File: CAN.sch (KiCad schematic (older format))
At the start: 9 parts, among them U7 MCP2542FDxMF

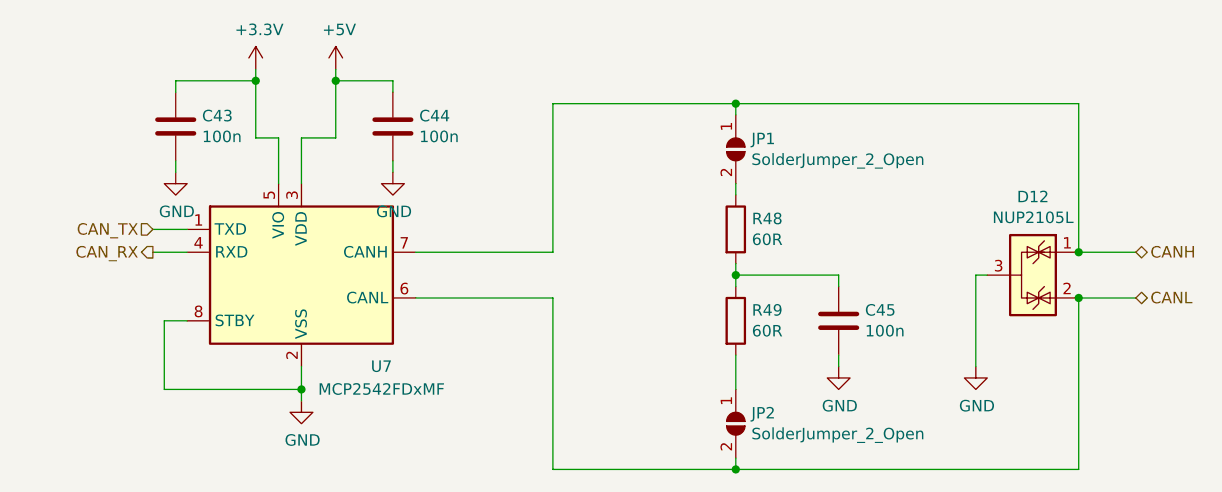
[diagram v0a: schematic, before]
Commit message: Added FET for LED
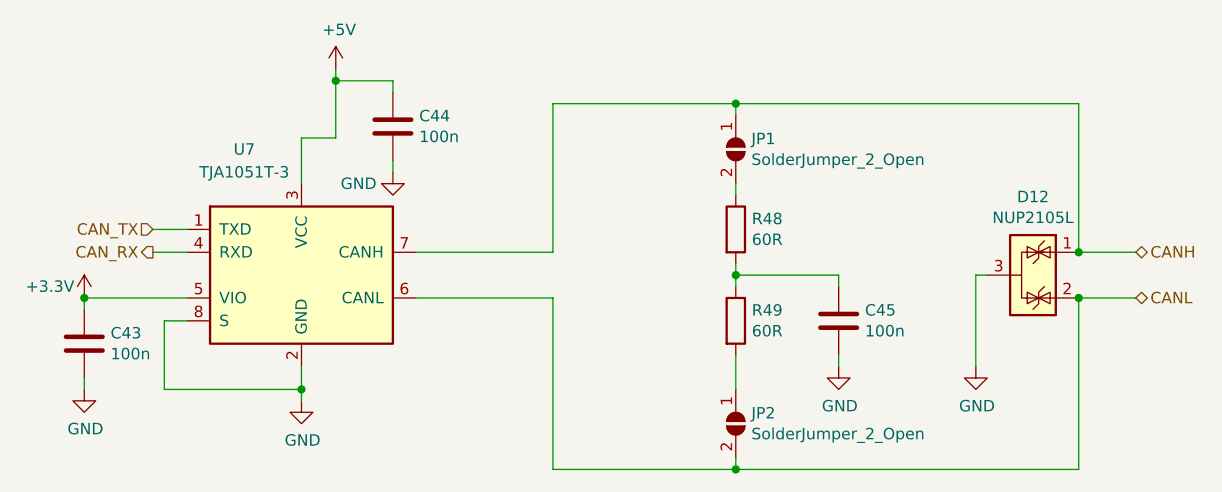
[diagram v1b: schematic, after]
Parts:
- removed U7: MCP2542FDxMF, Package_DFN_QFN:DFN-8-1EP_3x3mm_P0.65mm_EP1.55x2.4mm, symbol Interface_CAN_LIN:MCP2542FDxMF
- added U7: TJA1051T-3, Package_SO:SOIC-8_3.9x4.9mm_P1.27mm, symbol Interface_CAN_LIN:TJA1051T-3
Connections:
- net +3V3: now also U7.5 (VIO)
- net +5V: now also U7.3 (VCC)
- net CANH: now also U7.7 (CANH)
- net CANL: now also U7.6 (CANL)
- net CAN_RX: now also U7.4 (RXD)
- net CAN_TX: now also U7.1 (TXD)
- net GND: now also U7.2 (GND), U7.8 (S)
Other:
- moved on the sheet: C43
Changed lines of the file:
@@
 Comment4 ""
 $EndDescr
-$Comp
-L Interface_CAN_LIN:MCP2542FDxMF U7
-U 1 1 5F738629
-P 4750 3600
-F 0 "U7" H 5100 3200 50  0000 C CNN
-F 1 "MCP2542FDxMF" H 5100 3100 50  0000 C CNN
-F 2 "Package_DFN_QFN:DFN-8-1EP_3x3mm_P0.65mm_EP1.55x2.4mm" H 4750 3100 50  0001 C CIN
-F 3 "http://ww1.microchip.com/downloads/en/DeviceDoc/MCP2542FD-4FD-MCP2542WFD-4WFD-Data-Sheet20005514B.pdf" H 4750 3600 50  0001 C CNN
-	1    4750 3600
-	1    0    0    -1
-$EndComp
 Wire Wire Line
 	5250 3500 5850 3500
@@
 L power:+3.3V #PWR0228
 U 1 1 5F74847C
-P 4550 2700
-F 0 "#PWR0228" H 4550 2550 50  0001 C CNN
-F 1 "+3.3V" H 4565 2873 50  0000 C CNN
-F 2 "" H 4550 2700 50  0001 C CNN
-F 3 "" H 4550 2700 50  0001 C CNN
-	1    4550 2700
-	1    0    0    -1
-$EndComp
-Wire Wire Line
-	4550 2700 4550 2750
-Wire Wire Line
-	4550 3000 4650 3000
+P 3800 3700
+F 0 "#PWR0228" H 3800 3550 50  0001 C CNN
+F 1 "+3.3V" H 3650 3750 50  0000 C CNN
+F 2 "" H 3800 3700 50  0001 C CNN
+F 3 "" H 3800 3700 50  0001 C CNN
+	1    3800 3700
+	1    0    0    -1
+$EndComp
 $Comp
 L power:+5V #PWR0229
@@
 L Device:C C43
 U 1 1 5F74BE20
-P 4200 2950
-F 0 "C43" H 4315 2996 50  0000 L CNN
-F 1 "100n" H 4315 2905 50  0000 L CNN
-F 2 "Capacitor_SMD:C_0603_1608Metric" H 4238 2800 50  0001 C CNN
-F 3 "~" H 4200 2950 50  0001 C CNN
-	1    4200 2950
-	1    0    0    -1
-$EndComp
-Wire Wire Line
-	4200 2800 4200 2750
-Connection ~ 4550 2750
-Wire Wire Line
-	4550 2750 4550 3000
-Wire Wire Line
-	4200 3100 4200 3150
-Wire Wire Line
-	4200 2750 4550 2750
+P 3800 3900
+F 0 "C43" H 3915 3946 50  0000 L CNN
+F 1 "100n" H 3915 3855 50  0000 L CNN
+F 2 "Capacitor_SMD:C_0603_1608Metric" H 3838 3750 50  0001 C CNN
+F 3 "~" H 3800 3900 50  0001 C CNN
+	1    3800 3900
+	1    0    0    -1
+$EndComp
+Wire Wire Line
+	3800 3750 3800 3700
+Wire Wire Line
+	3800 4050 3800 4100
+Wire Wire Line
+	3800 3700 4250 3700
 $Comp
 L Device:C C44
@@
 	8150 3700 8400 3700
 Wire Wire Line
-	4650 3000 4650 3200
-Wire Wire Line
 	4750 3000 4750 3200
 $Comp
 L power:GND #PWR0222
 U 1 1 5F7D2541
-P 4200 3150
-F 0 "#PWR0222" H 4200 2900 50  0001 C CNN
-F 1 "GND" H 4205 2977 50  0000 C CNN
-F 2 "" H 4200 3150 50  0001 C CNN
-F 3 "" H 4200 3150 50  0001 C CNN
-	1    4200 3150
+P 3800 4100
+F 0 "#PWR0222" H 3800 3850 50  0001 C CNN
+F 1 "GND" H 3805 3927 50  0000 C CNN
+F 2 "" H 3800 4100 50  0001 C CNN
+F 3 "" H 3800 4100 50  0001 C CNN
+	1    3800 4100
 	1    0    0    -1
 $EndComp
@@
 P 5150 3150
 F 0 "#PWR0223" H 5150 2900 50  0001 C CNN
-F 1 "GND" H 5155 2977 50  0000 C CNN
+F 1 "GND" H 5000 3100 50  0000 C CNN
 F 2 "" H 5150 3150 50  0001 C CNN
 F 3 "" H 5150 3150 50  0001 C CNN
@@
 Wire Wire Line
 	7700 3600 7750 3600
+$Comp
+L Interface_CAN_LIN:TJA1051T-3 U7
+U 1 1 603E3A3E
+P 4750 3600
+F 0 "U7" H 4500 4150 50  0000 C CNN
+F 1 "TJA1051T-3" H 4500 4050 50  0000 C CNN
+F 2 "Package_SO:SOIC-8_3.9x4.9mm_P1.27mm" H 4750 3100 50  0001 C CIN
+F 3 "http://www.nxp.com/documents/data_sheet/TJA1051.pdf" H 4750 3600 50  0001 C CNN
+	1    4750 3600
+	1    0    0    -1
+$EndComp
+Connection ~ 3800 3700
 $EndSCHEMATC
